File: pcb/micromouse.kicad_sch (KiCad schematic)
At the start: 15 parts, among them J1 AVR-ISP-6, U1 TSSP77038ETR, U2 TSSP77038ETR, U3 TSSP77038ETR, U4 TSSP77038ETR, U5 TSSP77038ETR, U6 TSSP77038ETR, U7 ATmega328PB-A, U8 MX1508, Y1 Crystal

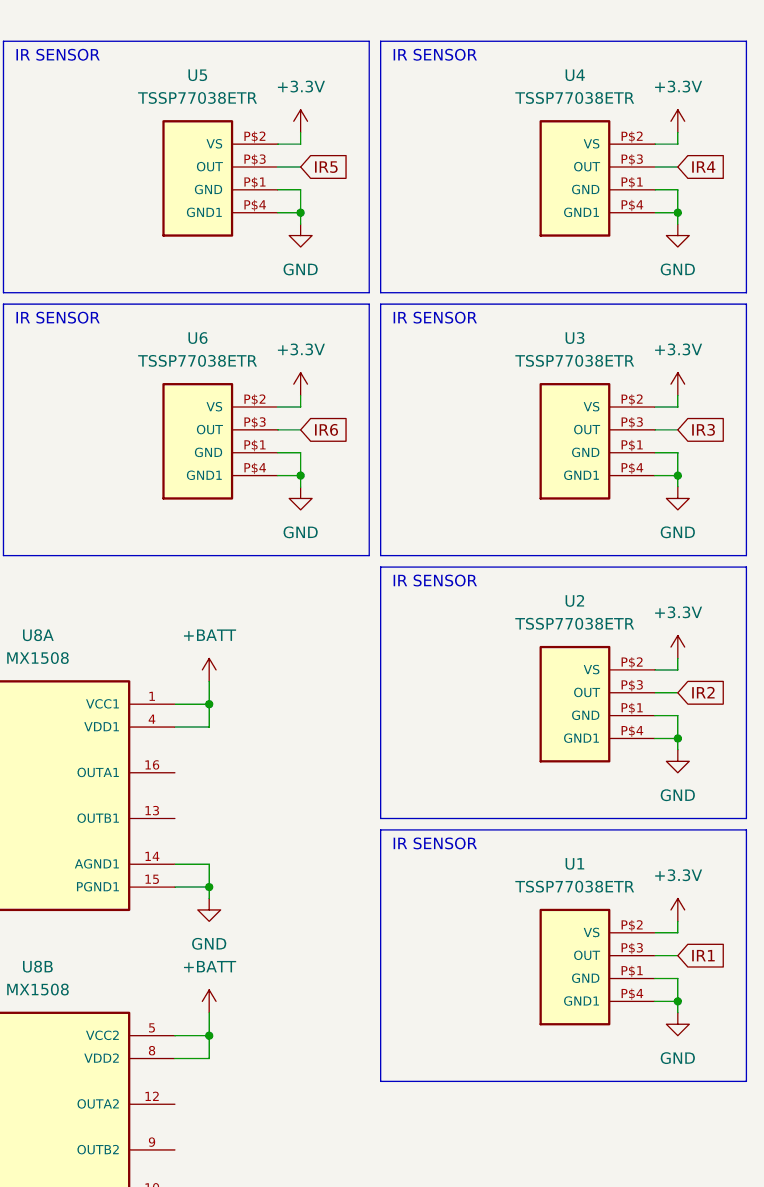
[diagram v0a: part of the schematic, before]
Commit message: wiring mcu
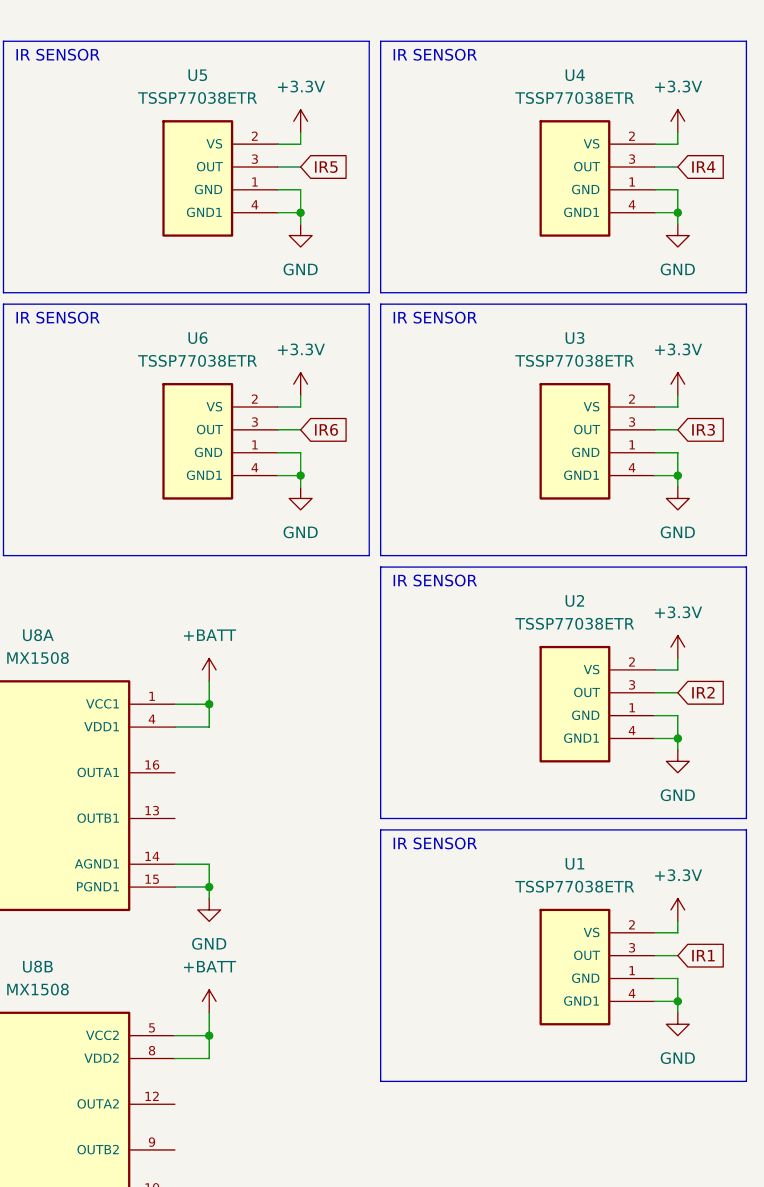
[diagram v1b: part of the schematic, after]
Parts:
- C1, C2, C3, C4, C5: footprint (none) -> Capacitor_SMD:C_0603_1608Metric
- J1: footprint (none) -> Connector_IDC:IDC-Header_2x03_P2.54mm_Horizontal
- U1, U2, U3, U4, U5, U6: footprint TSSP77038ETR:TSSP770 -> Library:TSSP77
- Y1: footprint (none) -> Crystal:Crystal_SMD_HC49-SD
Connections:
- net +3.3V: now also U1.2 (VS), U2.2 (VS), U3.2 (VS), U4.2 (VS), U5.2 (VS), U6.2 (VS); no longer U1.P$2 (VS), U2.P$2 (VS), U3.P$2 (VS), U4.P$2 (VS), U5.P$2 (VS), U6.P$2 (VS)
- net GND: now also U1.1 (GND), U1.4 (GND1), U2.1 (GND), U2.4 (GND1), U3.1 (GND), U3.4 (GND1), U4.1 (GND), U4.4 (GND1), U5.1 (GND), U5.4 (GND1), U6.1 (GND), U6.4 (GND1); no longer U1.P$1 (GND), U1.P$4 (GND1), U2.P$1 (GND), U2.P$4 (GND1), U3.P$1 (GND), U3.P$4 (GND1), U4.P$1 (GND), U4.P$4 (GND1), U5.P$1 (GND), U5.P$4 (GND1), U6.P$1 (GND), U6.P$4 (GND1)
- net IR1: now also U1.3 (OUT); no longer U1.P$3 (OUT)
- net IR2: now also U2.3 (OUT); no longer U2.P$3 (OUT)
- net IR3: now also U3.3 (OUT); no longer U3.P$3 (OUT)
- net IR4: now also U4.3 (OUT); no longer U4.P$3 (OUT)
- net IR5: now also U5.3 (OUT); no longer U5.P$3 (OUT)
- net IR6: now also U6.3 (OUT); no longer U6.P$3 (OUT)
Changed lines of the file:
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@@
       (effects (font (size 1.27 1.27)))
     )
-    (property "Footprint" "TSSP77038ETR:TSSP770" (at 224.79 58.42 0)
+    (property "Footprint" "Library:TSSP77" (at 224.79 58.42 0)
       (effects (font (size 1.27 1.27)) (justify bottom) hide)
     )
@@
       (effects (font (size 1.27 1.27)) (justify bottom) hide)
     )
-    (pin "P$1")
-    (pin "P$2")
-    (pin "P$3")
-    (pin "P$4")
+    (pin "1")
+    (pin "2")
+    (pin "3")
+    (pin "4")
     (instances
       (project "micromouse"
@@
       (effects (font (size 1.27 1.27)))
     )
-    (property "Footprint" "" (at 147.32 36.83 0)
+    (property "Footprint" "Capacitor_SMD:C_0603_1608Metric" (at 147.32 36.83 0)
       (effects (font (size 1.27 1.27)) hide)
     )
@@
       (effects (font (size 1.27 1.27)) (justify left))
     )
-    (property "Footprint" "" (at 35.56 38.1 0)
+    (property "Footprint" "Capacitor_SMD:C_0603_1608Metric" (at 35.56 38.1 0)
       (effects (font (size 1.27 1.27)) hide)
     )
@@
       (effects (font (size 1.27 1.27)) (justify left))
     )
-    (property "Footprint" "" (at 27.94 38.1 0)
+    (property "Footprint" "Capacitor_SMD:C_0603_1608Metric" (at 27.94 38.1 0)
       (effects (font (size 1.27 1.27)) hide)
     )
@@
       (effects (font (size 1.27 1.27)))
     )
-    (property "Footprint" "" (at 179.07 20.32 90)
+    (property "Footprint" "Connector_IDC:IDC-Header_2x03_P2.54mm_Horizontal" (at 179.07 20.32 90)
       (effects (font (size 1.27 1.27)) hide)
     )
@@
       (effects (font (size 1.27 1.27)))
     )
-    (property "Footprint" "TSSP77038ETR:TSSP770" (at 266.7 116.84 0)
+    (property "Footprint" "Library:TSSP77" (at 266.7 116.84 0)
       (effects (font (size 1.27 1.27)) (justify bottom) hide)
     )
@@
       (effects (font (size 1.27 1.27)) (justify bottom) hide)
     )
-    (pin "P$1")
-    (pin "P$2")
-    (pin "P$3")
-    (pin "P$4")
+    (pin "1")
+    (pin "2")
+    (pin "3")
+    (pin "4")
     (instances
       (project "micromouse"
@@
       (effects (font (size 1.27 1.27)) (justify left))
     )
-    (property "Footprint" "" (at 20.32 38.1 0)
+    (property "Footprint" "Capacitor_SMD:C_0603_1608Metric" (at 20.32 38.1 0)
       (effects (font (size 1.27 1.27)) hide)
     )
@@
       (effects (font (size 1.27 1.27)))
     )
-    (property "Footprint" "TSSP77038ETR:TSSP770" (at 266.7 58.42 0)
+    (property "Footprint" "Library:TSSP77" (at 266.7 58.42 0)
       (effects (font (size 1.27 1.27)) (justify bottom) hide)
     )
@@
       (effects (font (size 1.27 1.27)) (justify bottom) hide)
     )
-    (pin "P$1")
-    (pin "P$2")
-    (pin "P$3")
-    (pin "P$4")
+    (pin "1")
+    (pin "2")
+    (pin "3")
+    (pin "4")
     (instances
       (project "micromouse"
@@
       (effects (font (size 1.27 1.27)))
     )
-    (property "Footprint" "TSSP77038ETR:TSSP770" (at 266.7 29.21 0)
+    (property "Footprint" "Library:TSSP77" (at 266.7 29.21 0)
       (effects (font (size 1.27 1.27)) (justify bottom) hide)
     )
@@
       (effects (font (size 1.27 1.27)) (justify bottom) hide)
     )
-    (pin "P$1")
-    (pin "P$2")
-    (pin "P$3")
-    (pin "P$4")
+    (pin "1")
+    (pin "2")
+    (pin "3")
+    (pin "4")
     (instances
       (project "micromouse"
@@
       (effects (font (size 1.27 1.27)))
     )
-    (property "Footprint" "TSSP77038ETR:TSSP770" (at 266.7 87.63 0)
+    (property "Footprint" "Library:TSSP77" (at 266.7 87.63 0)
       (effects (font (size 1.27 1.27)) (justify bottom) hide)
     )
@@
       (effects (font (size 1.27 1.27)) (justify bottom) hide)
     )
-    (pin "P$1")
-    (pin "P$2")
-    (pin "P$3")
-    (pin "P$4")
+    (pin "1")
+    (pin "2")
+    (pin "3")
+    (pin "4")
     (instances
       (project "micromouse"
@@
       (effects (font (size 1.27 1.27)))
     )
-    (property "Footprint" "TSSP77038ETR:TSSP770" (at 224.79 29.21 0)
+    (property "Footprint" "Library:TSSP77" (at 224.79 29.21 0)
       (effects (font (size 1.27 1.27)) (justify bottom) hide)
     )
@@
       (effects (font (size 1.27 1.27)) (justify bottom) hide)
     )
-    (pin "P$1")
-    (pin "P$2")
-    (pin "P$3")
-    (pin "P$4")
+    (pin "1")
+    (pin "2")
+    (pin "3")
+    (pin "4")
     (instances
       (project "micromouse"
@@
       (effects (font (size 1.27 1.27)) (justify right))
     )
-    (property "Footprint" "" (at 139.7 29.21 0)
+    (property "Footprint" "Crystal:Crystal_SMD_HC49-SD" (at 139.7 29.21 0)
       (effects (font (size 1.27 1.27)) hide)
     )
@@
       (effects (font (size 1.27 1.27)))
     )
-    (property "Footprint" "" (at 147.32 22.86 0)
-      (effects (font (size 1.27 1.27)) hide)
-    )
+    (property "Footprint" "Capacitor_SMD:C_0603_1608Metric" (at 147.32 22.86 0)
+      (effects (font (size 1.27 1.27)) hide)
+    )
